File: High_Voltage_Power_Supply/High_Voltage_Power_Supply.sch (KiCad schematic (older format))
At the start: 96 parts, among them J1 Conn_01x02_Female, J2 Conn_01x02_Female, J3 Conn_01x02_Female, J4 Conn_01x12_Female, Q1 Q_NMOS_GDS, Q2 Q_NMOS_GDS, Q3 Q_NMOS_GDS, Q4 Q_NIGBT_GCE, U1 LT3751-TSSOP, U10 ADR3412, U11 LM2576HVT-15, U2 LT3751-TSSOP, U3 ZXGD3004E6, U4 ZXGD3004E6, U5 MC14504B, U6 MC14504B, U7 LM7805, U8 LM7805, U9 LMV331

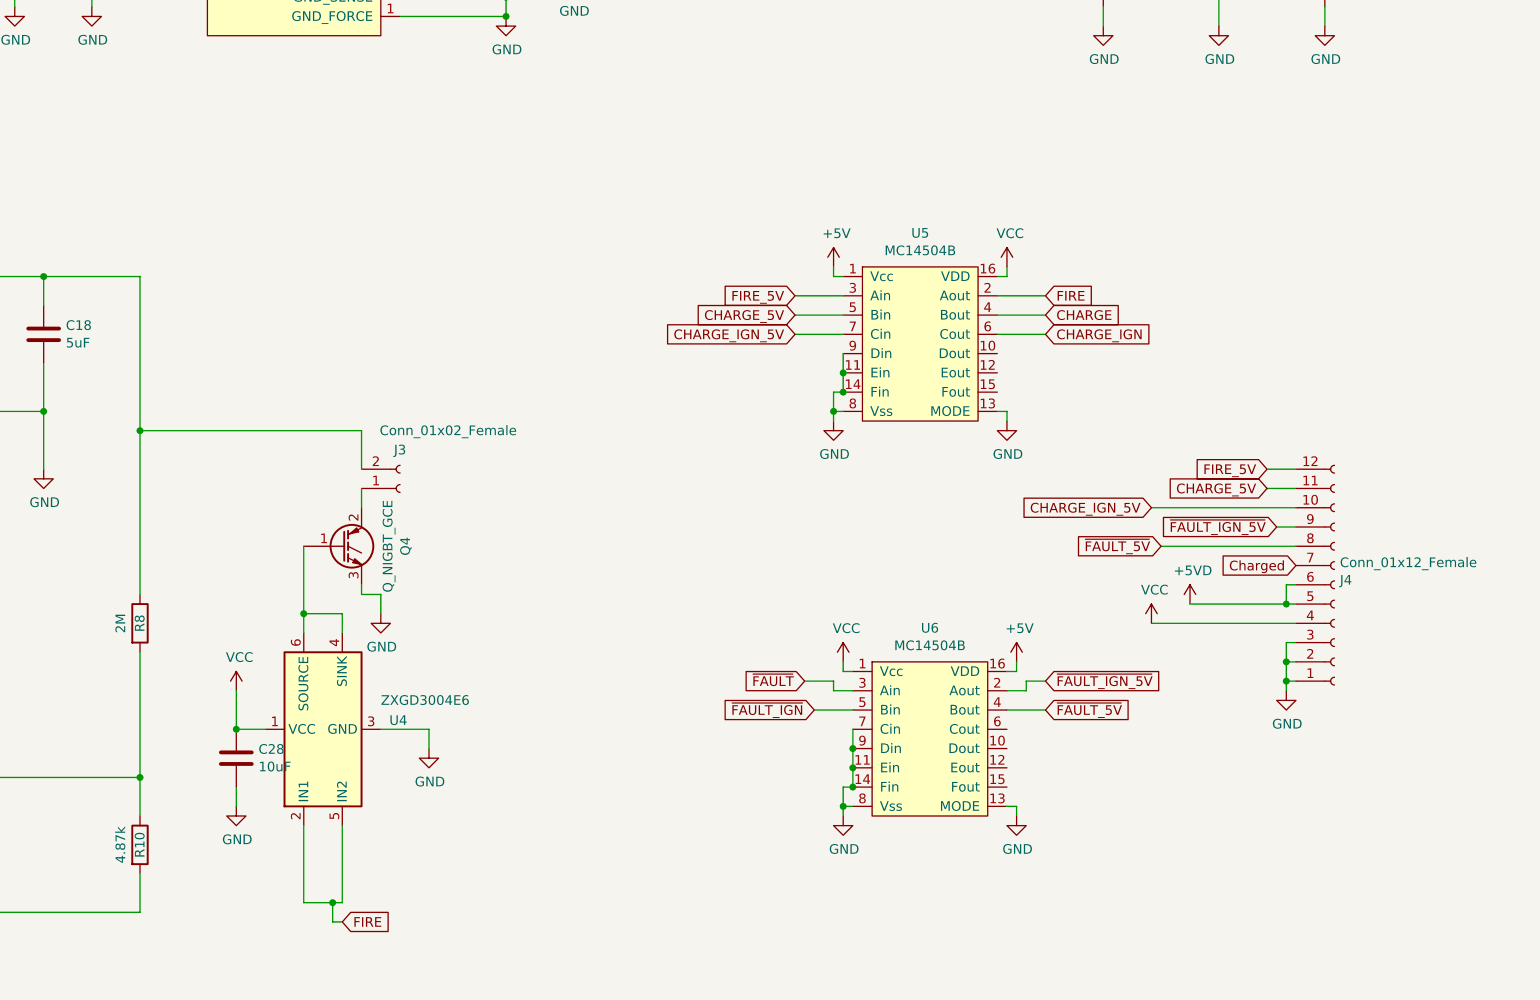
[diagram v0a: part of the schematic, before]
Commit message: updated BOM
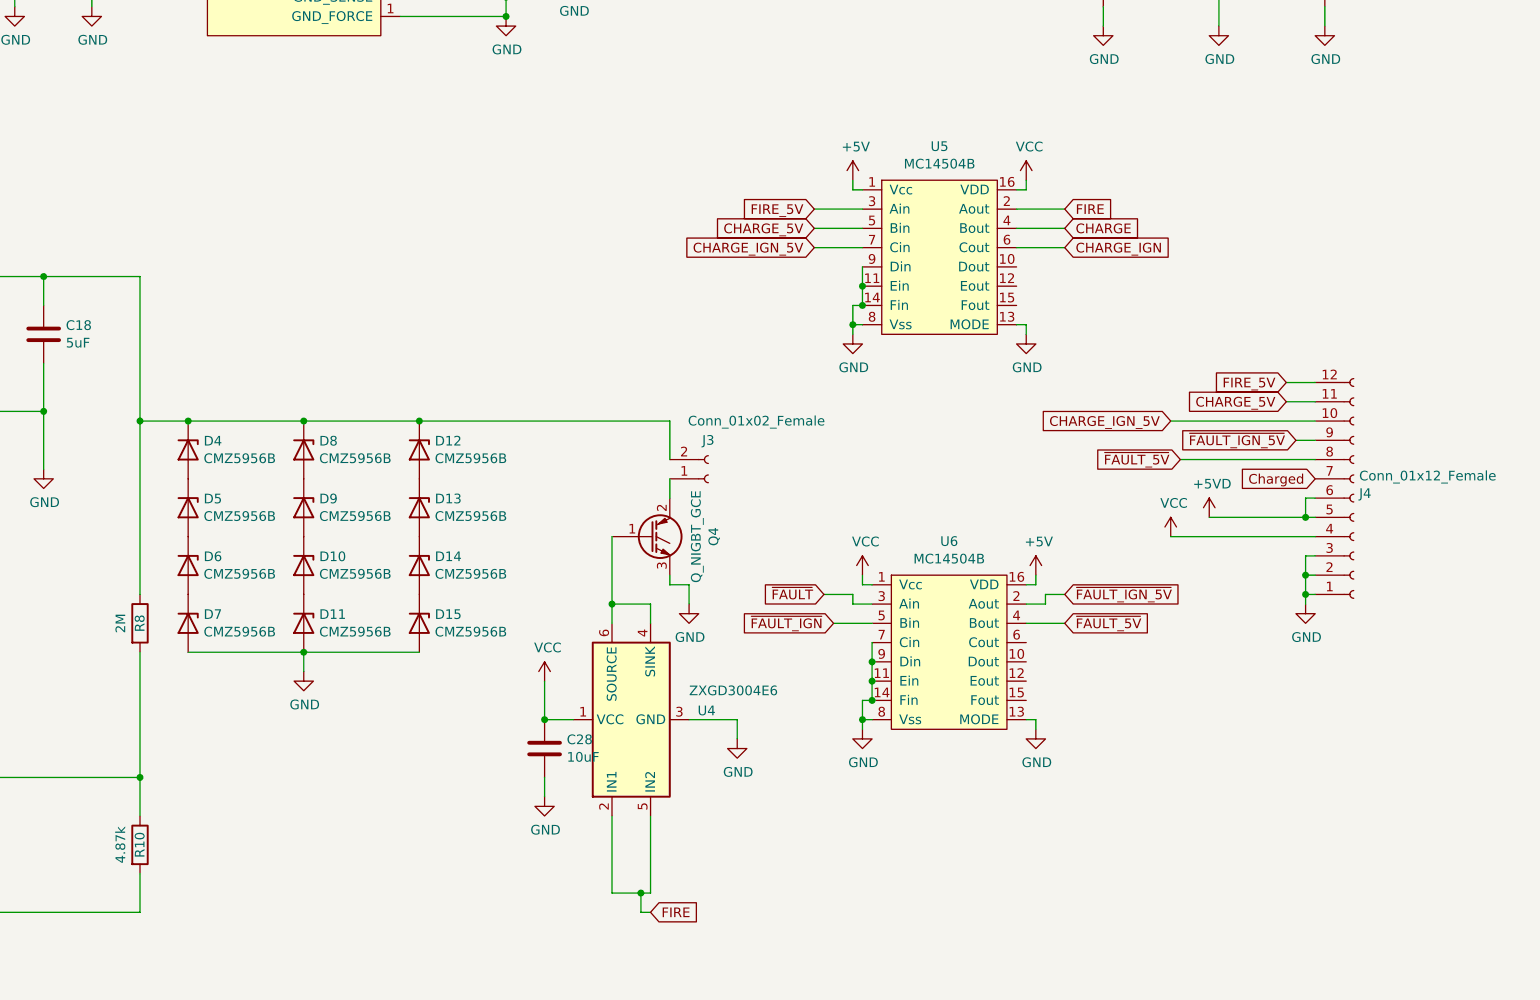
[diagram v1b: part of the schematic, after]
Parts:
- added D10, D11, D12, D13, D14, D15, D4, D5, D6, D7, D8, D9: CMZ5956B, Diode_SMD:D_SMA, symbol Device:D_Zener
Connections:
- net GND: now also D11.2 (A), D15.2 (A), D7.2 (A)
- net at C18.1, D2.1 (K), J3.2 (Pin_2)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: now also D12.1 (K), D4.1 (K), D8.1 (K)
- new net: D4.2 (A), D5.1 (K)
- new net: D5.2 (A), D6.1 (K)
- new net: D6.2 (A), D7.1 (K)
- new net: D8.2 (A), D9.1 (K)
- new net: D10.1 (K), D9.2 (A)
- new net: D10.2 (A), D11.1 (K)
- new net: D12.2 (A), D13.1 (K)
- new net: D13.2 (A), D14.1 (K)
- new net: D14.2 (A), D15.1 (K)
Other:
- moved on the sheet: C28, J3, J4, Q4, U4, U5, U6
